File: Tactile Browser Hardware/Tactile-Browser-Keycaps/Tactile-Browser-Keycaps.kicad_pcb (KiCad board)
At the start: 2 copper layers, 23.5 x 19 mm, 3 parts, among them J1 Conn_01x01_Pin, J2 Conn_01x01_Pin, SW1 SW_Push

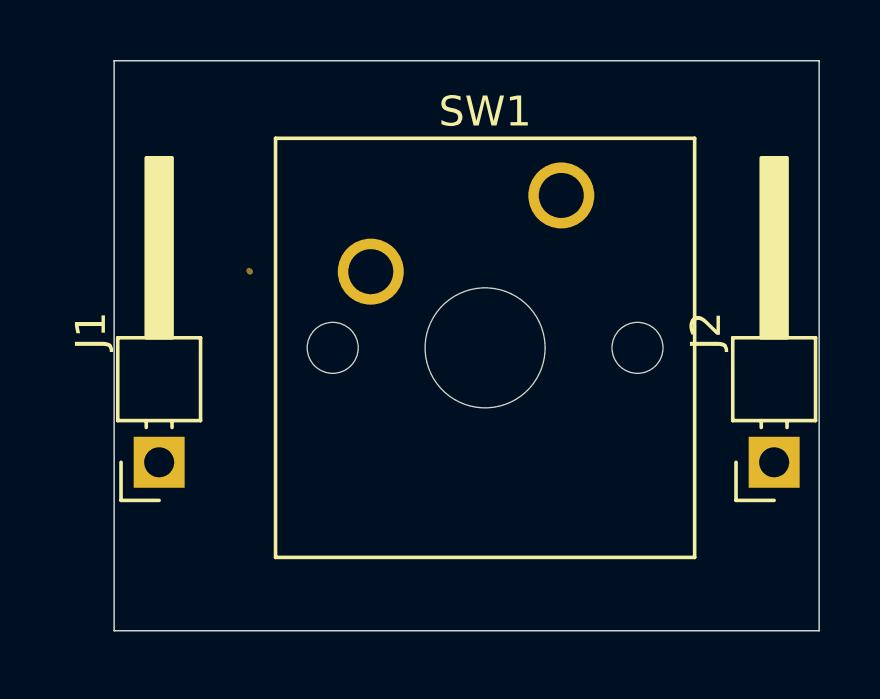
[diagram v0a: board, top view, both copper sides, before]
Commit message: ketyswitch
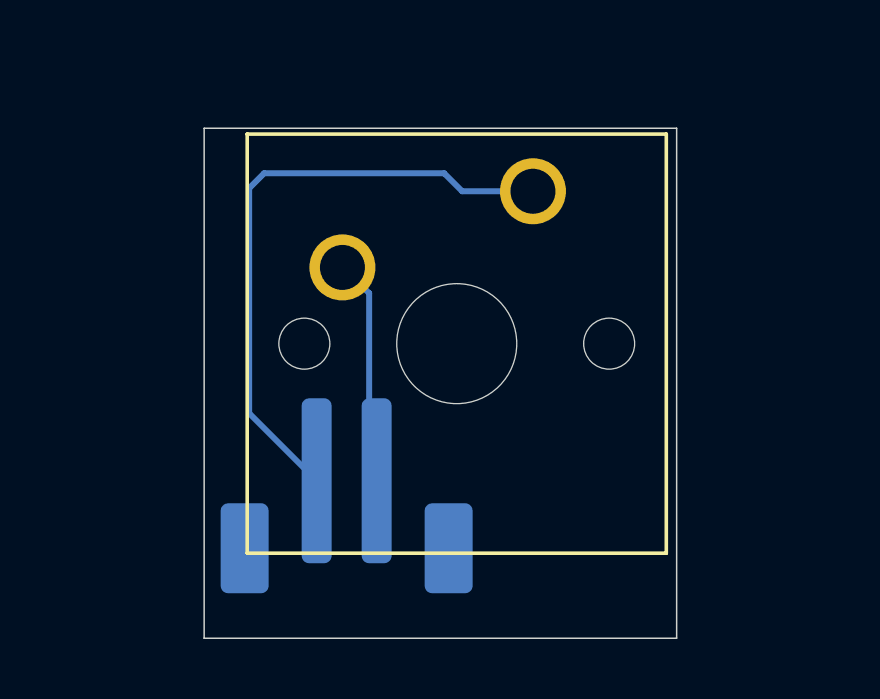
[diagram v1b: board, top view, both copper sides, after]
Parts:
- removed J2: Conn_01x01_Pin, Connector_PinHeader_2.54mm:PinHeader_1x01_P2.54mm_Horizontal
- J1: value Conn_01x01_Pin -> Conn_01x02_Pin; footprint Connector_PinHeader_2.54mm:PinHeader_1x01_P2.54mm_Horizontal -> Connector_JST:JST_PH_B2B-PH-SM4-TB_1x02-1MP_P2.00mm_Vertical; moved to B.Cu
- moved J1 6.35 mm to (103.8, 101.5), turned to 0 degrees
- moved SW1 0.96 mm to (110.0, 91.3)
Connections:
- SW1 pad 1: Net-(J2-Pin_1) -> Net-(J1-Pin_1)
- SW1 pad 2: Net-(J1-Pin_1) -> Net-(J1-Pin_2)
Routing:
- net Net-(J1-Pin_1): track 0.04 -> 20.6 mm
- net Net-(J1-Pin_2): track 0.00 -> 7.50 mm
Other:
- board size 23.5 x 19 mm -> 15.8 x 17 mm
